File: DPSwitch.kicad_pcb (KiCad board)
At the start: 4 copper layers, 71 x 74.5 mm, 43 parts, among them J1 USB_OTG, J2 USB_OTG, J3 DP_47272, J4 DP_47272, J5 DP_47272, J6 USB_A, SW1 SEL_A, SW2 SEL_B, U1 HD3SS215, U2 74LVC2G00DC, U3 MCP1700-3302E_SOT23

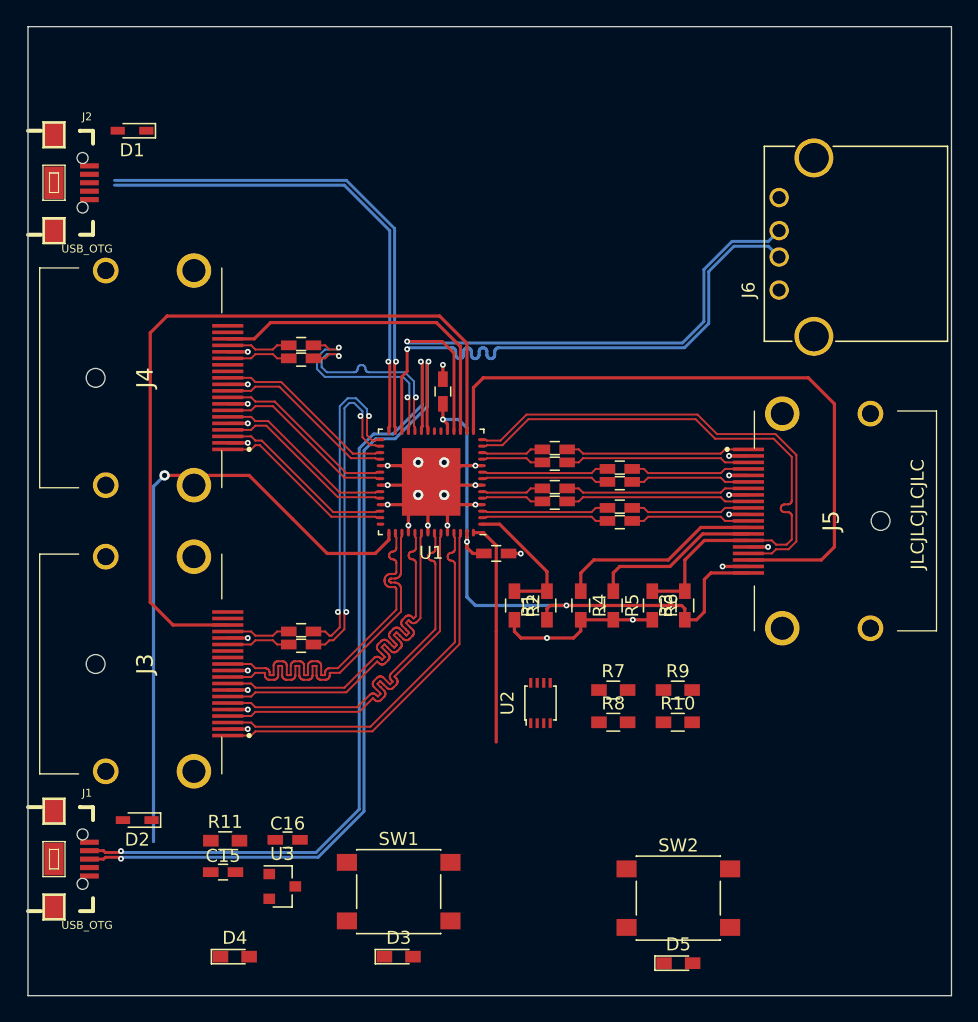
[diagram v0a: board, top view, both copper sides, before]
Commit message: Rev1 for manufacture
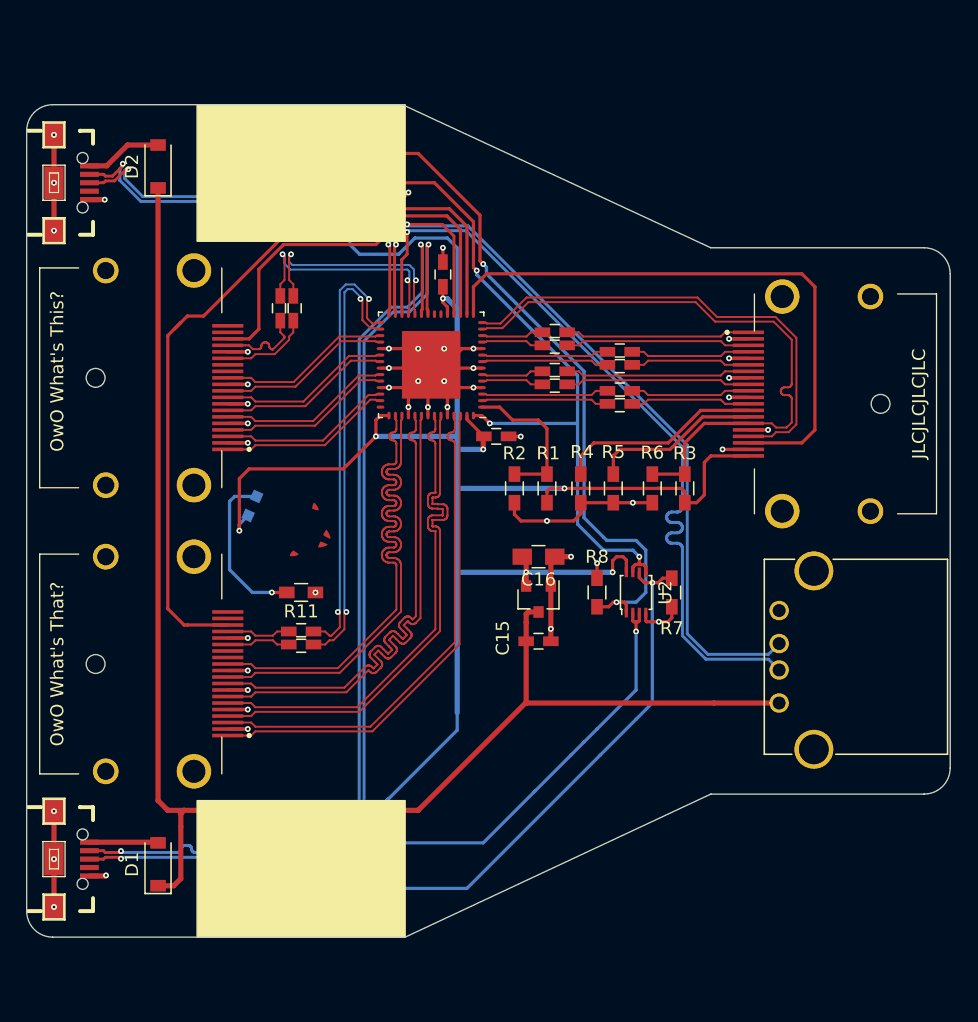
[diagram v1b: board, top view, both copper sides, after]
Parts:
- C16: footprint Capacitors_SMD:C_0603_HandSoldering -> Capacitors_SMD:C_0805_HandSoldering
- D1, D2: value D_Small -> BAT54GWJ; footprint Diodes_SMD:D_SC-80_HandSoldering -> Diodes_SMD:D_SOD-123
- D4: footprint LEDs:LED_0603_HandSoldering -> Visclib:wolfpaw-0.3-illuminated
- moved D5 64.7 mm to (87.4, 46.5), turned to 270 degrees
- moved SW2 63.2 mm to (80.3, 46.5), turned to 180 degrees
- moved D1 56.4 mm to (71.5, 98.9), turned to 90 degrees
- moved D2 50.3 mm to (71.5, 45.2), turned to 90 degrees
- moved R9 44.8 mm to (89.5, 46.5), turned to 90 degrees
- moved D4 33.5 mm to (81.8, 72.8), turned to 270 degrees
- moved J6 31.8 mm to (119.2, 86.5)
- moved C15 30.1 mm to (100.8, 81.8), turned to 180 degrees
- moved U3 29.6 mm to (100.8, 78.5), turned to 270 degrees
- moved C16 29.1 mm to (100.8, 75.2), turned to 180 degrees
- moved R10 24.1 mm to (89.8, 98.5), turned to 90 degrees
- moved R11 20.0 mm to (82.5, 78.0), turned to 180 degrees
- moved U2 11.2 mm to (108.2, 78.0)
- moved R8 10.1 mm to (105.2, 78.0), turned to 90 degrees
- moved SW1 9.92 mm to (80.4, 98.5)
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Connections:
- J1 pad 1: Net-(D2-Pad2) -> Net-(D1-Pad2)
- J2 pad 1: Net-(D1-Pad2) -> Net-(D2-Pad2)
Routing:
- net VDD: track 0.00 -> 113.8 mm
- net +3V3: track 97.8 -> 164.3 mm, vias 4 -> 9
- net /SW_B: track 0.00 -> 63.6 mm, vias 0 -> 2
- net /SW_A: track 0.00 -> 53.1 mm, vias 0 -> 2
- net /DX_SEL: track 17.3 -> 53.3 mm, vias 0 -> 3
- net /~Q: track 0.00 -> 34.3 mm, vias 0 -> 2
- net GND: track 60.3 -> 93.1 mm, vias 33 -> 48
- net /UC_P: track 44.5 -> 61.1 mm
- net /UC_N: track 44.5 -> 61.1 mm
- net Net-(D4-Pad1): track 0.00 -> 12.6 mm, vias 0 -> 1
- net /UB_N: track 65.0 -> 74.5 mm
- net /DA3_P: track 29.1 -> 38.3 mm
- net /DA3_N: track 29.1 -> 38.4 mm
- net /DA1_N: track 29.3 -> 38.5 mm
- net /DA1_P: track 29.2 -> 38.4 mm
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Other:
- board size 71 x 74.5 mm -> 71 x 64 mm
- board text added: "OwO What's That?"
- board text added: "OwO What's This?"
